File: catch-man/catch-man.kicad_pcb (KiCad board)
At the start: 2 copper layers, 108.8 x 118.5 mm, 24 parts, among them Q1 2N3904, SW1 SW_Push_45deg, SW2 SW_SPDT, U1 STC8G1K08A-36I-DFN8

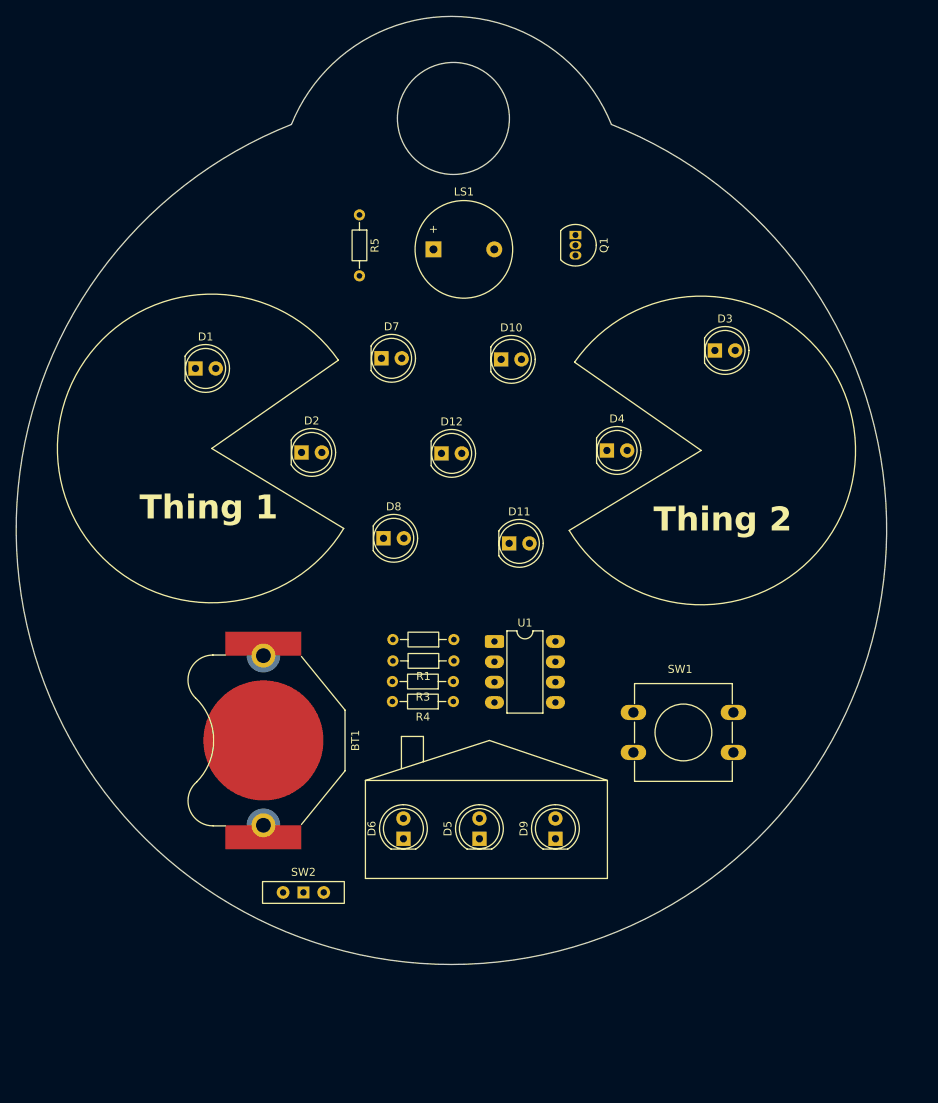
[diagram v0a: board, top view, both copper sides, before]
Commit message: catch-man: v1
Finished layout, centered parts
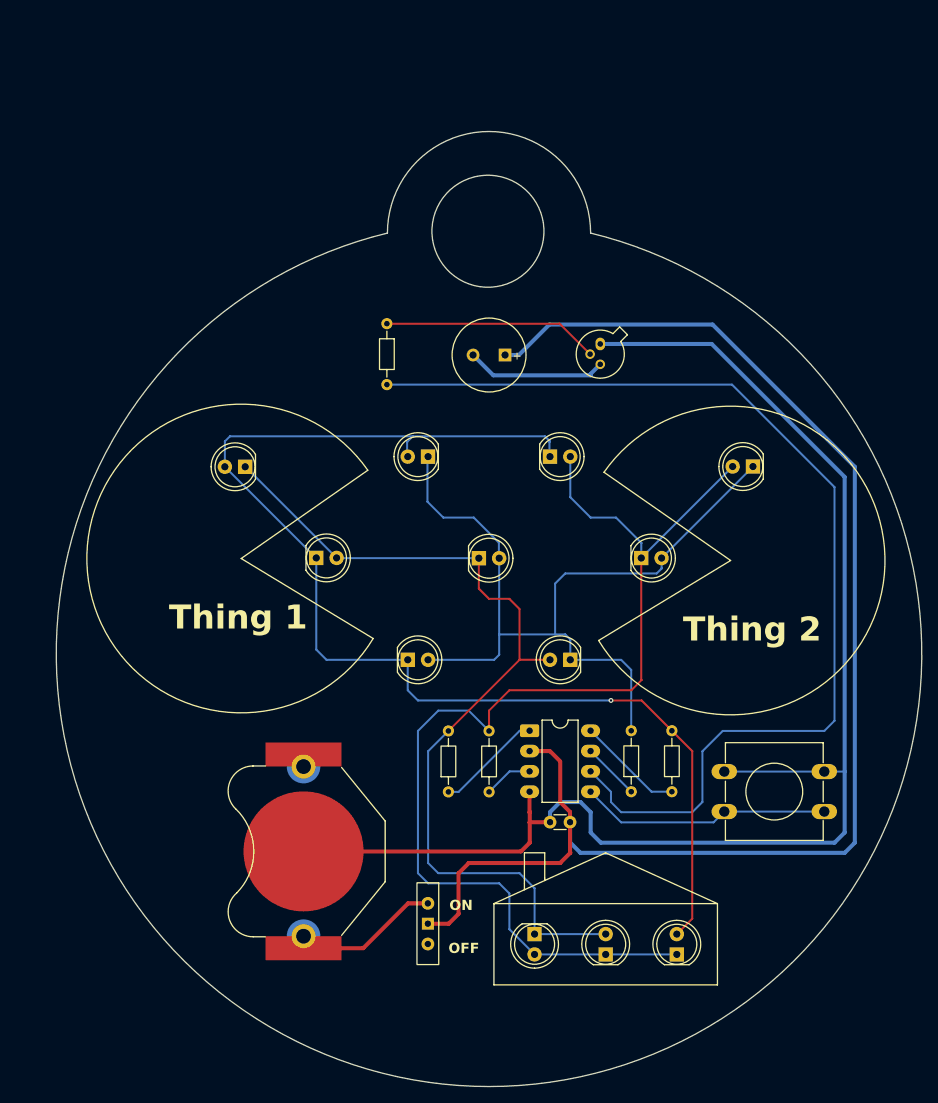
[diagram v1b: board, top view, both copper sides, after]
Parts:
- added C1: 0.1u, Capacitor_THT:C_Disc_D3.0mm_W1.6mm_P2.50mm, F.Cu at (149.8, 142.2)
- LS1: value Speaker -> 9024 Passive Buzzer; footprint Buzzer_Beeper:Buzzer_12x9.5RM7.6 -> Buzzer_Beeper:MagneticBuzzer_PUI_AT-0927-TT-6-R
- Q1: value 2N3904 -> 2N2222; footprint Package_TO_SOT_THT:TO-92_Inline -> Package_TO_SOT_THT:TO-18-3
- SW2: value SW_SPDT -> POWER
- U1: value STC8G1K08A-36I-DFN8 -> STC8G1K08A-36I-DIP8
- moved R1 31.8 mm to (162.6, 138.4), turned to 90 degrees
- moved R4 24.9 mm to (157.5, 138.4), turned to 90 degrees
- moved D5 21.4 mm to (154.3, 158.7)
- moved D9 21.0 mm to (163.2, 158.7)
- moved D6 20.3 mm to (145.4, 156.2), turned to -90 degrees
- moved R2 19.1 mm to (134.6, 138.4), turned to 90 degrees
- moved D11 16.4 mm to (149.9, 121.9), turned to 180 degrees
- moved SW2 16.0 mm to (132.1, 154.9), turned to -90 degrees
- moved LS1 16.0 mm to (141.7, 83.8), turned to 180 degrees
- moved D8 15.5 mm to (129.5, 121.9)
- moved D3 15.3 mm to (172.7, 97.8), turned to 180 degrees
- moved BT1 14.7 mm to (116.5, 145.9)
- moved R3 14.5 mm to (139.7, 138.4), turned to 90 degrees
- moved D4 14.1 mm to (158.7, 109.2)
- moved R5 14.0 mm to (126.9, 79.9)
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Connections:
- net Net-(SW2-A) renamed /VCC
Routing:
- net /VCC: track 0.00 -> 179.6 mm
- net GND: track 0.00 -> 177.3 mm
- net Net-(D1-A): track 0.00 -> 154.8 mm, vias 0 -> 1
- net Net-(D10-A): track 0.00 -> 140.8 mm
- net Net-(U1-P3.1): track 0.00 -> 132.3 mm
- net Net-(D1-K): track 0.00 -> 113.4 mm
- net Net-(D11-K): track 0.00 -> 105.2 mm
- net Net-(U1-P3.0): track 0.00 -> 31.4 mm
- net Net-(Q1-B): track 0.00 -> 27.0 mm
- net Net-(BT1-+): track 0.00 -> 17.9 mm
- net Net-(Q1-C): track 0.00 -> 17.6 mm
- net Net-(U1-P3.3): track 0.00 -> 13.3 mm
- net Net-(U1-P5.4): track 0.00 -> 13.3 mm
- net Net-(U1-P3.2): track 0.00 -> 7.19 mm
- net Net-(U1-P5.5): track 0.00 -> 6.13 mm
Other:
- board size 108.8 x 118.5 mm -> 108.2 x 119.4 mm
- board text added: "OFF"
- board text added: "ON"
